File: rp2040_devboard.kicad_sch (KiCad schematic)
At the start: 25 parts, among them J1 USB_C_Receptacle_USB2.0_14P, U1 RP2040, U2 NCP1117-3.3_SOT223, Y1 12MHz

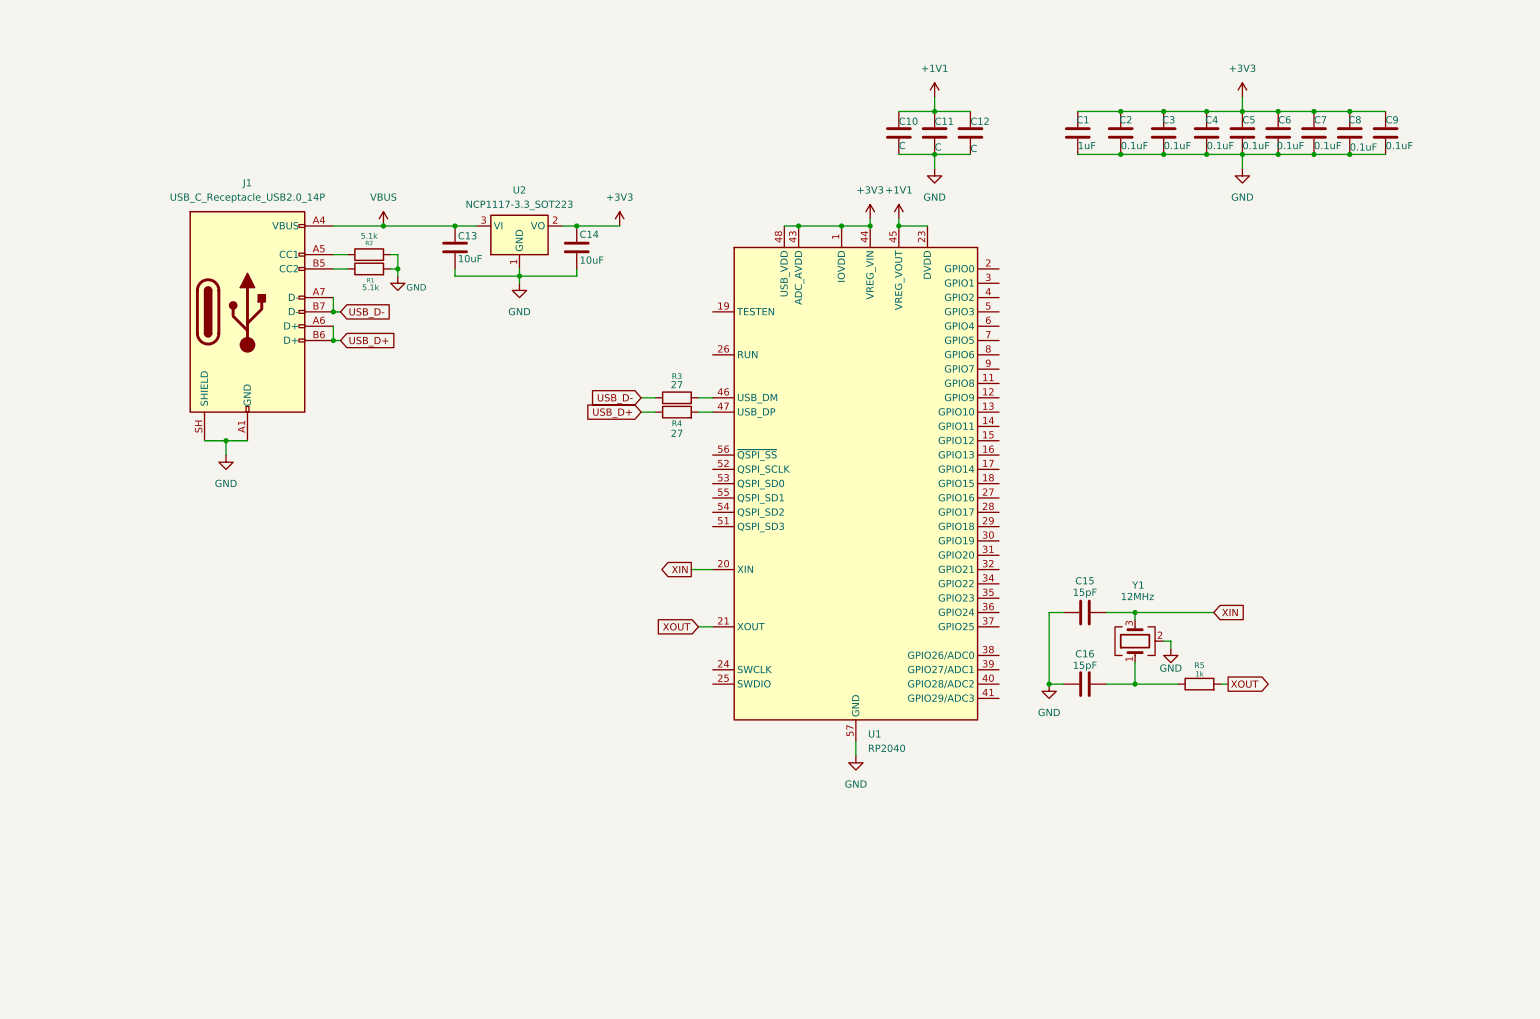
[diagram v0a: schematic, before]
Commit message: almost finished the schematic
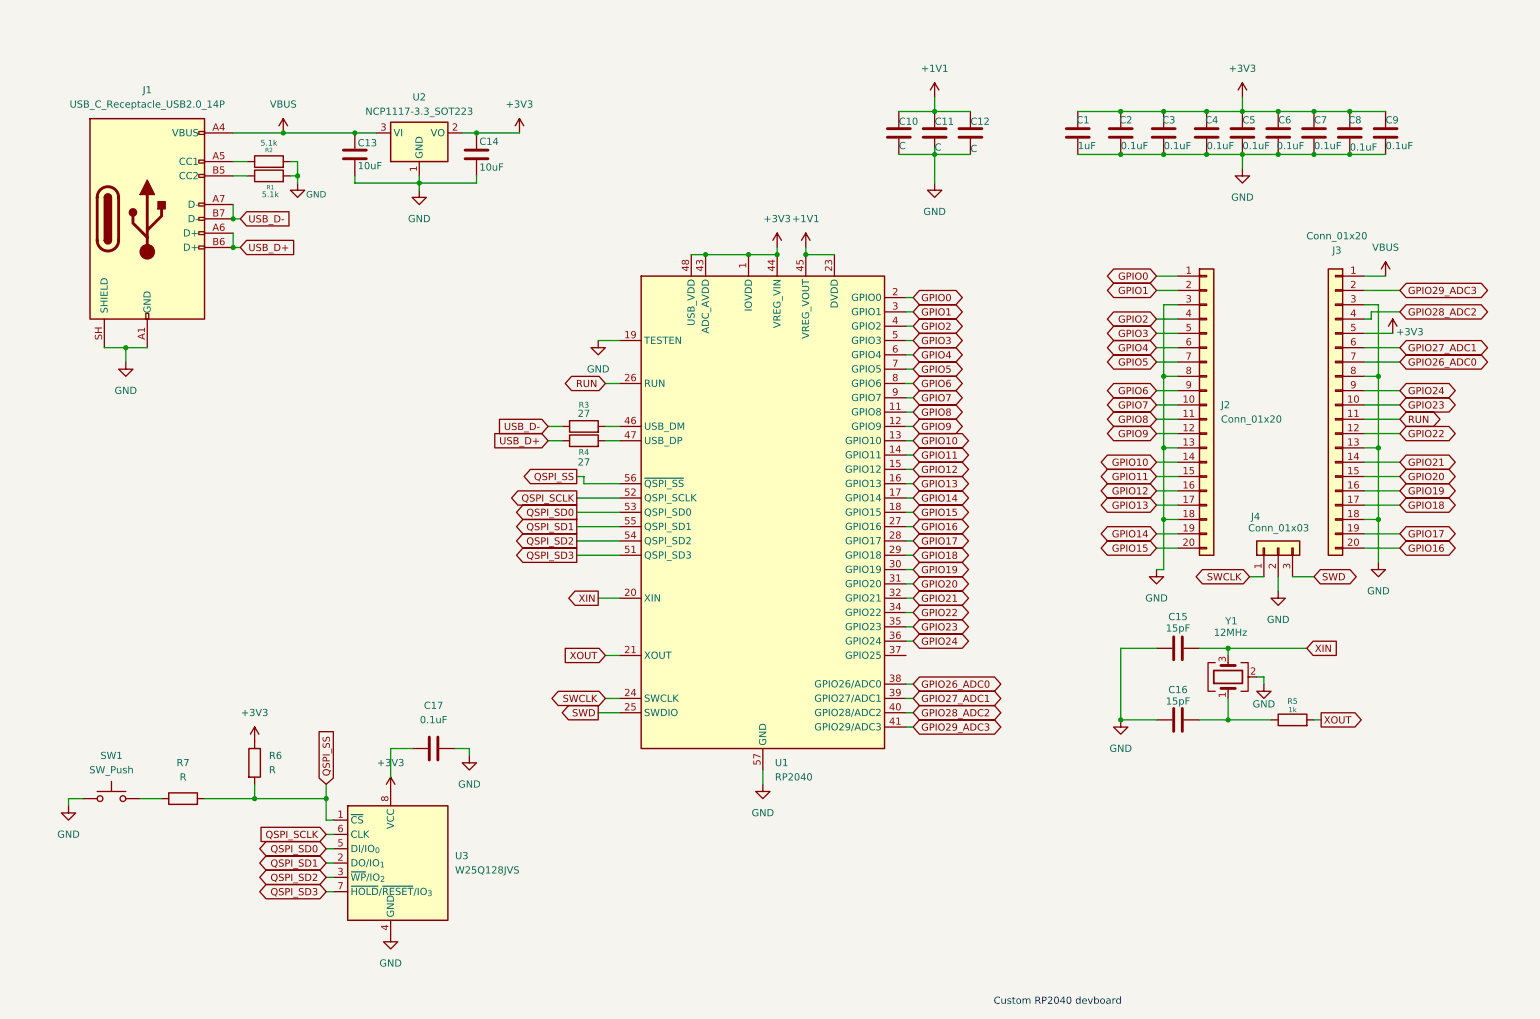
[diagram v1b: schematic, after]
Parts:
- added C17: 0.1uF, symbol Device:C
- added J2, J3: Conn_01x20, symbol Connector_Generic:Conn_01x20
- added J4: Conn_01x03, symbol Connector_Generic:Conn_01x03
- added R6, R7: R, symbol Device:R
- added SW1: SW_Push, symbol Switch:SW_Push
- added U3: W25Q128JVS, Package_SO:SOIC-8_5.3x5.3mm_P1.27mm, symbol Memory_Flash:W25Q128JVS
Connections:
- net +3V3: now also J3.5 (Pin_5), R6.1, U3.8 (VCC)
- net GND: now also U1.19 (TESTEN), C17.1, J2.13 (Pin_13), J2.18 (Pin_18), J2.3 (Pin_3), J2.8 (Pin_8), J3.13 (Pin_13), J3.18 (Pin_18), J3.3 (Pin_3), J3.8 (Pin_8), J4.2 (Pin_2), SW1.1, U3.4 (GND)
- net VBUS: now also J3.1 (Pin_1)
- net GPIO8: now reaches U1.11 (GPIO8)
- net GPIO8: now also J2.11 (Pin_11)
- net GPIO9: now reaches U1.12 (GPIO9)
- net GPIO9: now also J2.12 (Pin_12)
- net GPIO10: now reaches U1.13 (GPIO10)
- net GPIO10: now also J2.14 (Pin_14)
- net GPIO11: now reaches U1.14 (GPIO11)
- net GPIO11: now also J2.15 (Pin_15)
- net GPIO12: now reaches U1.15 (GPIO12)
- net GPIO12: now also J2.16 (Pin_16)
- net GPIO13: now reaches U1.16 (GPIO13)
- net GPIO13: now also J2.17 (Pin_17)
- net GPIO14: now reaches U1.17 (GPIO14)
- net GPIO14: now also J2.19 (Pin_19)
- net GPIO15: now reaches U1.18 (GPIO15)
- net GPIO15: now also J2.20 (Pin_20)
- net GPIO0: now reaches U1.2 (GPIO0)
- net GPIO0: now also J2.1 (Pin_1)
- net SWCLK: now reaches U1.24 (SWCLK)
- net SWCLK: now also J4.1 (Pin_1)
- net SWD: now reaches U1.25 (SWDIO)
- net SWD: now also J4.3 (Pin_3)
- net RUN: now reaches U1.26 (RUN)
- net RUN: now also J3.11 (Pin_11)
- net GPIO16: now reaches U1.27 (GPIO16)
- net GPIO16: now also J3.20 (Pin_20)
- net GPIO17: now reaches U1.28 (GPIO17)
- net GPIO17: now also J3.19 (Pin_19)
- net GPIO18: now reaches U1.29 (GPIO18)
- net GPIO18: now also J3.17 (Pin_17)
- net GPIO1: now reaches U1.3 (GPIO1)
- net GPIO1: now also J2.2 (Pin_2)
- net GPIO19: now reaches U1.30 (GPIO19)
- net GPIO19: now also J3.16 (Pin_16)
- net GPIO20: now reaches U1.31 (GPIO20)
- net GPIO20: now also J3.15 (Pin_15)
- net GPIO21: now reaches U1.32 (GPIO21)
- net GPIO21: now also J3.14 (Pin_14)
- net GPIO22: now reaches U1.34 (GPIO22)
- net GPIO22: now also J3.12 (Pin_12)
- net GPIO23: now reaches U1.35 (GPIO23)
- net GPIO23: now also J3.10 (Pin_10)
- net GPIO24: now reaches U1.36 (GPIO24)
- net GPIO24: now also J3.9 (Pin_9)
- net GPIO26_ADC0: now reaches U1.38 (GPIO26/ADC0)
- net GPIO26_ADC0: now also J3.7 (Pin_7)
- net GPIO27_ADC1: now reaches U1.39 (GPIO27/ADC1)
- net GPIO27_ADC1: now also J3.6 (Pin_6)
- net GPIO2: now reaches U1.4 (GPIO2)
- net GPIO2: now also J2.4 (Pin_4)
- net GPIO28_ADC2: now reaches U1.40 (GPIO28/ADC2)
- net GPIO28_ADC2: now also J3.4 (Pin_4)
- net GPIO29_ADC3: now reaches U1.41 (GPIO29/ADC3)
- net GPIO29_ADC3: now also J3.2 (Pin_2)
- net GPIO3: now reaches U1.5 (GPIO3)
- net GPIO3: now also J2.5 (Pin_5)
- net QSPI_SD3: now reaches U1.51 (QSPI_SD3)
- net QSPI_SD3: now also U3.7 (~{HOLD}/~{RESET}/IO_{3})
- net QSPI_SCLK: now reaches U1.52 (QSPI_SCLK)
- net QSPI_SCLK: now also U3.6 (CLK)
- net QSPI_SD0: now reaches U1.53 (QSPI_SD0)
- net QSPI_SD0: now also U3.5 (DI/IO_{0})
- net QSPI_SD2: now reaches U1.54 (QSPI_SD2)
- net QSPI_SD2: now also U3.3 (~{WP}/IO_{2})
- net QSPI_SD1: now reaches U1.55 (QSPI_SD1)
- net QSPI_SD1: now also U3.2 (DO/IO_{1})
- net QSPI_SS: now reaches U1.56 (~{QSPI_SS})
- net QSPI_SS: now also R6.2, R7.2, U3.1 (~{CS})
- net GPIO4: now reaches U1.6 (GPIO4)
- net GPIO4: now also J2.6 (Pin_6)
- net GPIO5: now reaches U1.7 (GPIO5)
- net GPIO5: now also J2.7 (Pin_7)
- net GPIO6: now reaches U1.8 (GPIO6)
- net GPIO6: now also J2.9 (Pin_9)
- net GPIO7: now reaches U1.9 (GPIO7)
- net GPIO7: now also J2.10 (Pin_10)
- new net: R7.1, SW1.2
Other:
- note added: "Custom RP2040 devboard"
- moved on the sheet: C13, C14, C15, C16, J1, R1, R2, R3, R4, R5, U1, U2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

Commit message: finished the schematic, added footprints
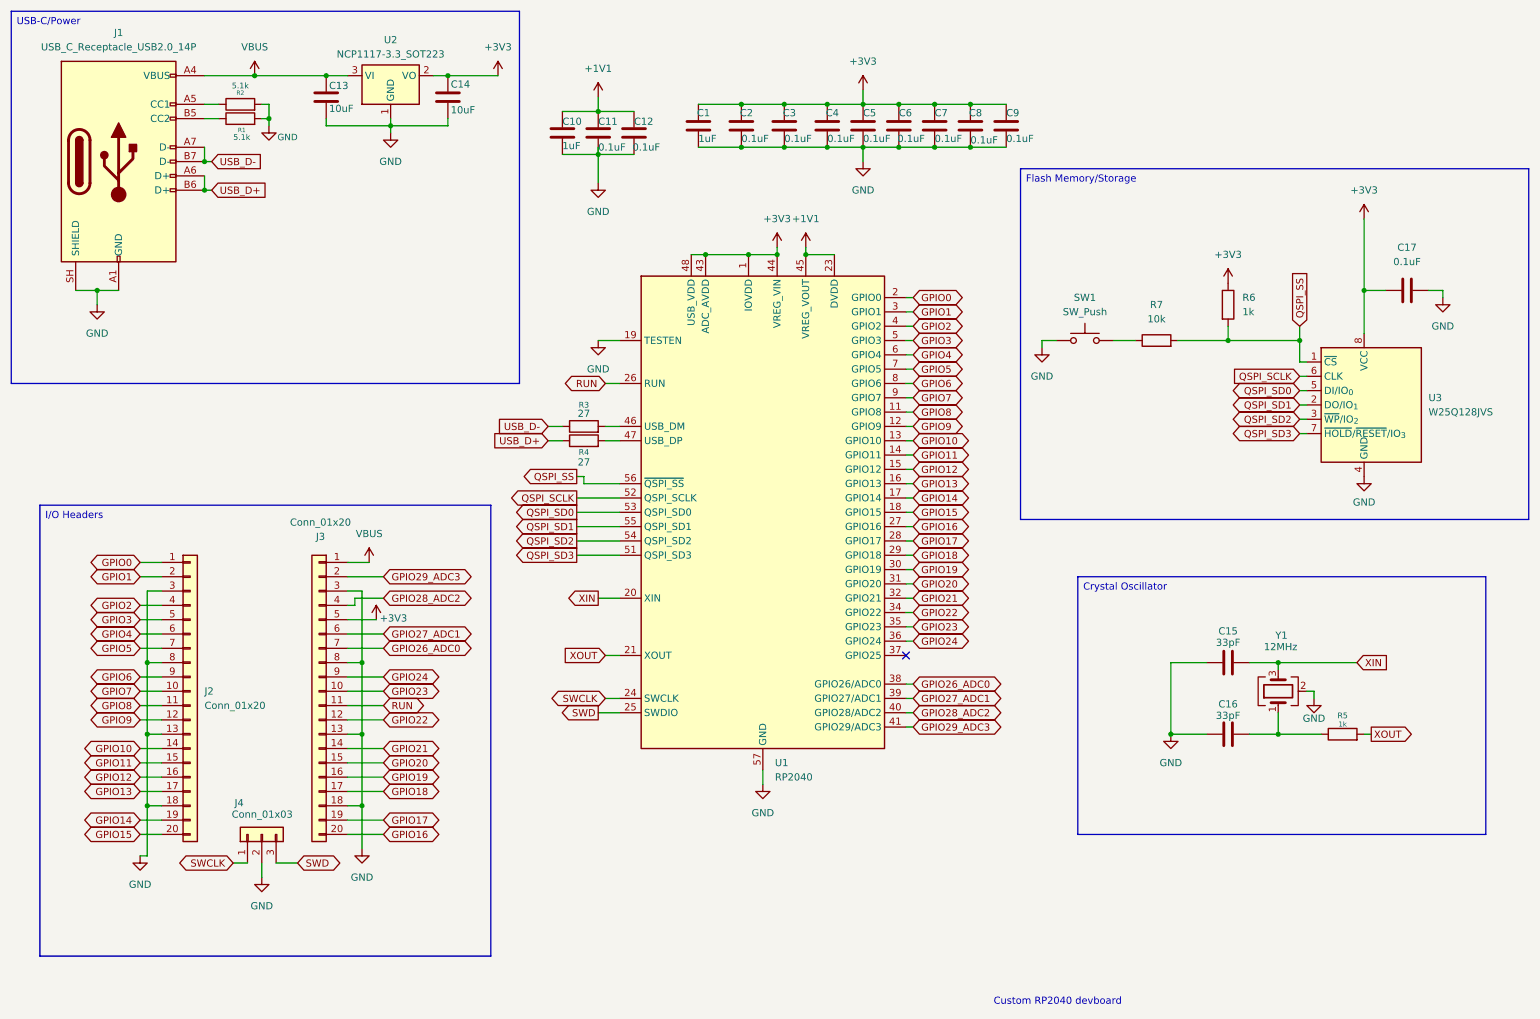
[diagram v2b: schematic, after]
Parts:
- C1, C17, C2, C3, C4, C5, C6, C7, C8, C9: footprint (none) -> Capacitor_SMD:C_0402_1005Metric
- C10: value C -> 1uF; footprint (none) -> Capacitor_SMD:C_0402_1005Metric
- C11, C12: value C -> 0.1uF; footprint (none) -> Capacitor_SMD:C_0402_1005Metric
- C13, C14: footprint (none) -> Capacitor_SMD:C_0603_1608Metric
- C15, C16: value 15pF -> 33pF; footprint (none) -> Capacitor_SMD:C_0402_1005Metric
- J1: footprint (none) -> Connector_USB:USB_C_Receptacle_HRO_TYPE-C-31-M-12
- J2, J3: footprint (none) -> Connector_PinHeader_2.54mm:PinHeader_1x20_P2.54mm_Vertical
- J4: footprint (none) -> Connector_PinHeader_2.54mm:PinHeader_1x03_P2.54mm_Vertical
- R1, R2, R3, R4, R5: footprint (none) -> Resistor_SMD:R_0402_1005Metric
- R6: value R -> 1k; footprint (none) -> Resistor_SMD:R_0402_1005Metric
- R7: value R -> 10k; footprint (none) -> Resistor_SMD:R_0402_1005Metric
- SW1: footprint (none) -> Button_Switch_SMD:SW_Push_SPST_NO_Alps_SKRK
- Y1: footprint (none) -> Crystal:Crystal_SMD_3225-4Pin_3.2x2.5mm
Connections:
- net +3V3: now also C17.2
- no-connect marks 0 -> 1
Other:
- moved on the sheet: C1, C10, C11, C12, C13, C14, C15, C16, C17, C2, C3, C4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

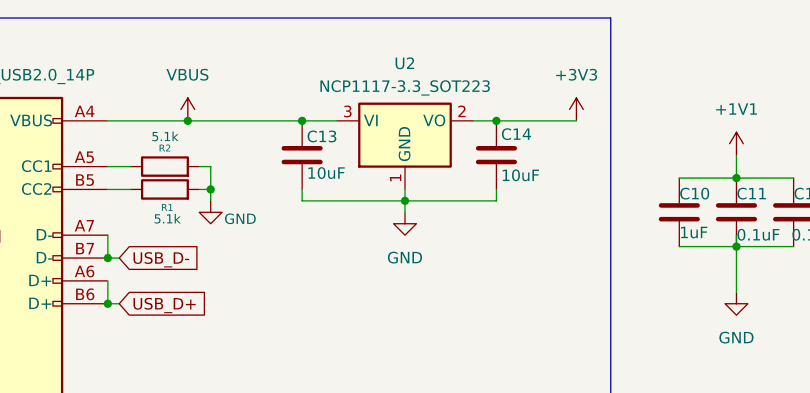
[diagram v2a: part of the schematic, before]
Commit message: starting the routing process
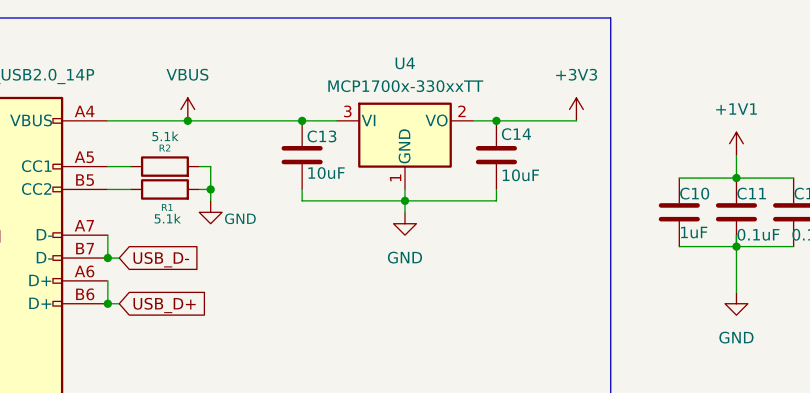
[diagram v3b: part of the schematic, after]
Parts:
- removed U2: NCP1117-3.3_SOT223, Package_TO_SOT_SMD:SOT-223-3_TabPin2, symbol Regulator_Linear:NCP1117-3.3_SOT223
- added U4: MCP1700x-330xxTT, Package_TO_SOT_SMD:SOT-23, symbol Regulator_Linear:MCP1700x-330xxTT
- U3: footprint Package_SO:SOIC-8_5.3x5.3mm_P1.27mm -> Package_SON:Winbond_USON-8-1EP_3x2mm_P0.5mm_EP0.2x1.6mm
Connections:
- net +3V3: now also U4.2 (VO)
- net GND: now also U4.1 (GND)
- net VBUS: now also U4.3 (VI)
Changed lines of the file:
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@@
+	)
+	(symbol
+		(lib_id "Regulator_Linear:MCP1700x-330xxTT")
+		(at 81.28 25.4 0)
+		(unit 1)
+		(body_style 1)
+		(exclude_from_sim no)
+		(in_bom yes)
+		(on_board yes)
+		(in_pos_files yes)
+		(dnp no)
+		(fields_autoplaced yes)
+		(property "Reference" "U4"
+			(at 81.28 19.05 0)
+			(show_name no)
+			(do_not_autoplace no)
+			(effects
+				(font
+					(size 1.27 1.27)
+				)
+			)
+		)
+		(property "Value" "MCP1700x-330xxTT"
+			(at 81.28 21.59 0)
+			(show_name no)
+			(do_not_autoplace no)
+			(effects
+				(font
+					(size 1.27 1.27)
+				)
+			)
+		)
+		(property "Footprint" "Package_TO_SOT_SMD:SOT-23"
+			(at 81.28 19.685 0)
+			(hide yes)
+			(show_name no)
+			(do_not_autoplace no)
+			(effects
+				(font
+					(size 1.27 1.27)
+				)
+			)
+		)
+		(property "Datasheet" "http://ww1.microchip.com/downloads/en/DeviceDoc/20001826D.pdf"
+			(at 81.28 25.4 0)
+			(hide yes)
+			(show_name no)
+			(do_not_autoplace no)
+			(effects
+				(font
+					(size 1.27 1.27)
+				)
+			)
+		)
+		(property "Description" "250mA Low Quiscent Current LDO, 3.3V output, SOT-23"
+			(at 81.28 25.4 0)
+			(hide yes)
+			(show_name no)
+			(do_not_autoplace no)
+			(effects
+				(font
+					(size 1.27 1.27)
+				)
+			)
+		)
+		(pin "3"
+		)
+		(pin "2"
+		)
+		(pin "1"
+		)
+		(instances
+			(project "rp2040_devboard"
+				(path "/8099f720-5a46-4059-82f0-4268e89e9a82"
+					(reference "U4")
+					(unit 1)
+				)
+			)
+		)
 	)
 	(symbol
@@
 	)
 	(symbol
-		(lib_id "Regulator_Linear:NCP1117-3.3_SOT223")
-		(at 81.28 25.4 0)
-		(unit 1)
-		(body_style 1)
-		(exclude_from_sim no)
-		(in_bom yes)
-		(on_board yes)
-		(in_pos_files yes)
-		(dnp no)
-		(fields_autoplaced yes)
-		(property "Reference" "U2"
-			(at 81.28 19.05 0)
-			(show_name no)
-			(do_not_autoplace no)
-			(effects
-				(font
-					(size 1.27 1.27)
-				)
-			)
-		)
-		(property "Value" "NCP1117-3.3_SOT223"
-			(at 81.28 21.59 0)
-			(show_name no)
-			(do_not_autoplace no)
-			(effects
-				(font
-					(size 1.27 1.27)
-				)
-			)
-		)
-		(property "Footprint" "Package_TO_SOT_SMD:SOT-223-3_TabPin2"
-			(at 81.28 20.32 0)
-			(hide yes)
-			(show_name no)
-			(do_not_autoplace no)
-			(effects
-				(font
-					(size 1.27 1.27)
-				)
-			)
-		)
-		(property "Datasheet" "http://www.onsemi.com/pub_link/Collateral/NCP1117-D.PDF"
-			(at 83.82 31.75 0)
-			(hide yes)
-			(show_name no)
-			(do_not_autoplace no)
-			(effects
-				(font
-					(size 1.27 1.27)
-				)
-			)
-		)
-		(property "Description" "1A Low drop-out regulator, Fixed Output 3.3V, SOT-223"
-			(at 81.28 25.4 0)
-			(hide yes)
-			(show_name no)
-			(do_not_autoplace no)
-			(effects
-				(font
-					(size 1.27 1.27)
-				)
-			)
-		)
-		(pin "3"
-		)
-		(pin "2"
-		)
-		(pin "1"
-		)
-		(instances
-			(project "rp2040_devboard"
-				(path "/8099f720-5a46-4059-82f0-4268e89e9a82"
-					(reference "U2")
-					(unit 1)
-				)
-			)
-		)
-	)
-	(symbol
 		(lib_id "Connector_Generic:Conn_01x03")
 		(at 58.42 160.02 90)
@@
 			)
 		)
-		(property "Footprint" "Package_SO:SOIC-8_5.3x5.3mm_P1.27mm"
+		(property "Footprint" "Package_SON:Winbond_USON-8-1EP_3x2mm_P0.5mm_EP0.2x1.6mm"
 			(at 254 60.96 0)
 			(hide yes)
